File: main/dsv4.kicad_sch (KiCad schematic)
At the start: 3 parts, among them J101 Conn_01x02, J102 Conn_01x02, J103 Conn_01x02

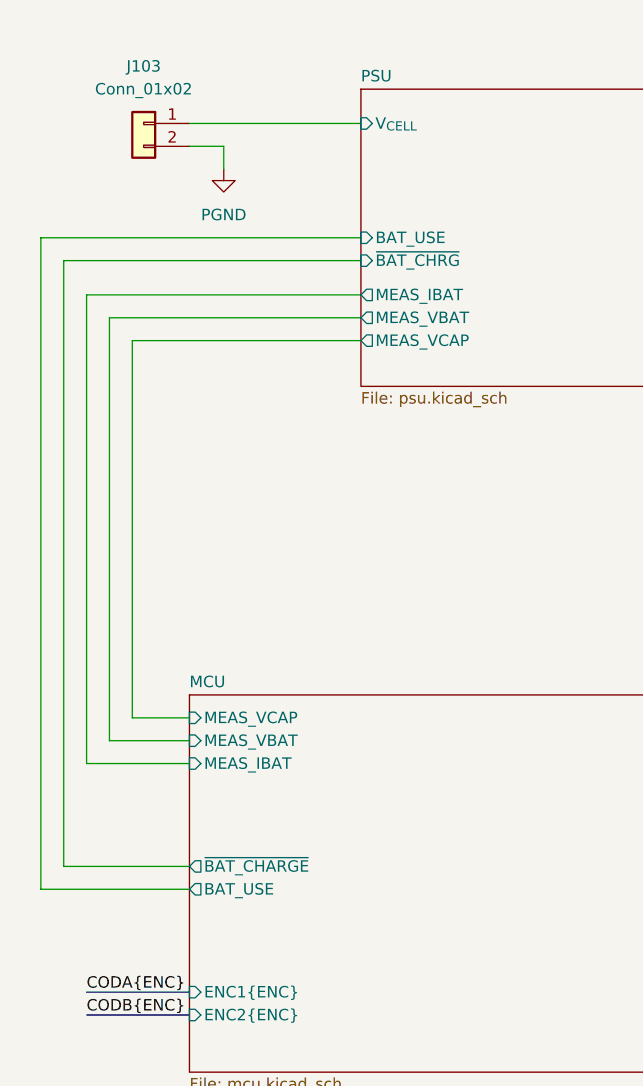
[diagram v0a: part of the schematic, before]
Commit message: Route of power rails
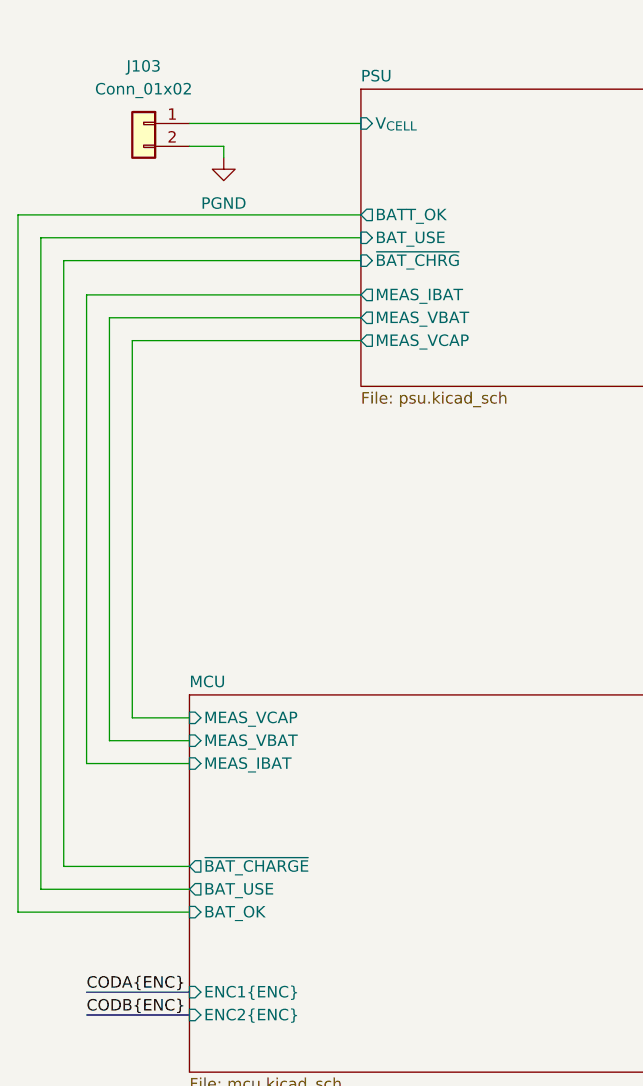
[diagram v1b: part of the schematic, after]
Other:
- sheet MCU ports: added BAT_OK; removed none
- sheet PSU ports: added BATT_OK; removed none
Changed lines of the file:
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@@
+	(wire
+		(pts
+			(xy 50.8 38.1) (xy 12.7 38.1)
+		)
+		(stroke
+			(width 0)
+			(type default)
+		)
+	)
 	(wire
 		(pts
@@
 	(wire
 		(pts
+			(xy 12.7 115.57) (xy 31.75 115.57)
+		)
+		(stroke
+			(width 0)
+			(type default)
+		)
+	)
+	(wire
+		(pts
 			(xy 50.8 46.99) (xy 20.32 46.99)
 		)
@@
 	(wire
 		(pts
+			(xy 12.7 38.1) (xy 12.7 115.57)
+		)
+		(stroke
+			(width 0)
+			(type default)
+		)
+	)
+	(wire
+		(pts
 			(xy 31.75 110.49) (xy 17.78 110.49)
 		)
@@
 	(wire
 		(pts
-			(xy 35.56 33.02) (xy 35.56 30.48)
+			(xy 35.56 31.75) (xy 35.56 30.48)
 		)
 		(stroke
@@
 	(symbol
 		(lib_id "power:GND")
-		(at 35.56 33.02 0)
+		(at 35.56 31.75 0)
 		(unit 1)
 		(exclude_from_sim no)
@@
 		(fields_autoplaced yes)
 		(property "Reference" "#PWR0104"
-			(at 35.56 39.37 0)
+			(at 35.56 38.1 0)
 			(effects
 				(font
@@
 		)
 		(property "Value" "PGND"
-			(at 35.56 38.1 0)
+			(at 35.56 36.83 0)
 			(effects
 				(font
@@
 		)
 		(property "Footprint" ""
-			(at 35.56 33.02 0)
+			(at 35.56 31.75 0)
 			(effects
 				(font
@@
 		)
 		(property "Datasheet" ""
-			(at 35.56 33.02 0)
+			(at 35.56 31.75 0)
 			(effects
 				(font
@@
 		)
 		(property "Description" "Power symbol creates a global label with name \"GND\" , ground"
-			(at 35.56 33.02 0)
+			(at 35.56 31.75 0)
 			(effects
 				(font
@@
 			)
 		)
+		(pin "BAT_OK" input
+			(at 31.75 115.57 180)
+			(effects
+				(font
+					(size 1.27 1.27)
+				)
+				(justify left)
+			)
+		)
 		(instances
 			(project "dsv4"
@@
 			(effects
 				(font
+					(size 1.27 1.27)
+				)
+				(justify left)
+			)
+		)
+		(pin "BATT_OK" output
+			(at 50.8 38.1 180)
+			(effects
+				(font
